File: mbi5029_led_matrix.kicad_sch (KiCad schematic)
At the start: 19 parts, among them Q1 pCh SO23, Q10 pCh SO23, Q11 pCh SO23, Q12 pCh SO23, Q13 pCh SO23, Q14 pCh SO23, Q15 pCh SO23, Q16 pCh SO23, Q2 pCh SO23, Q3 pCh SO23, Q4 pCh SO23, Q5 pCh SO23, Q6 pCh SO23, Q7 pCh SO23, Q8 pCh SO23, Q9 pCh SO23, U1 MBI5029, U2 74HC237, U3 74HC237

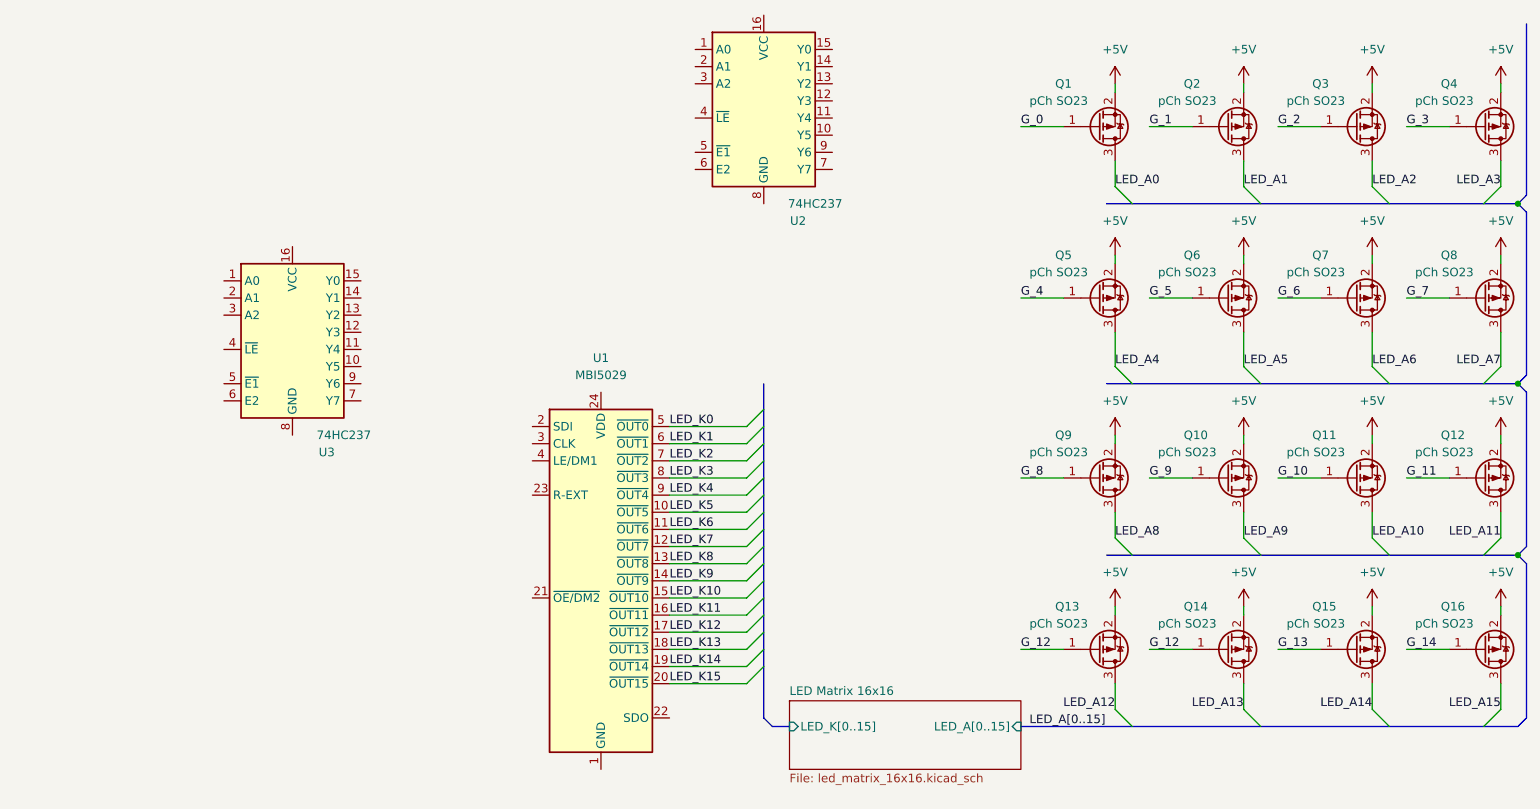
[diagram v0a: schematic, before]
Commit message: work
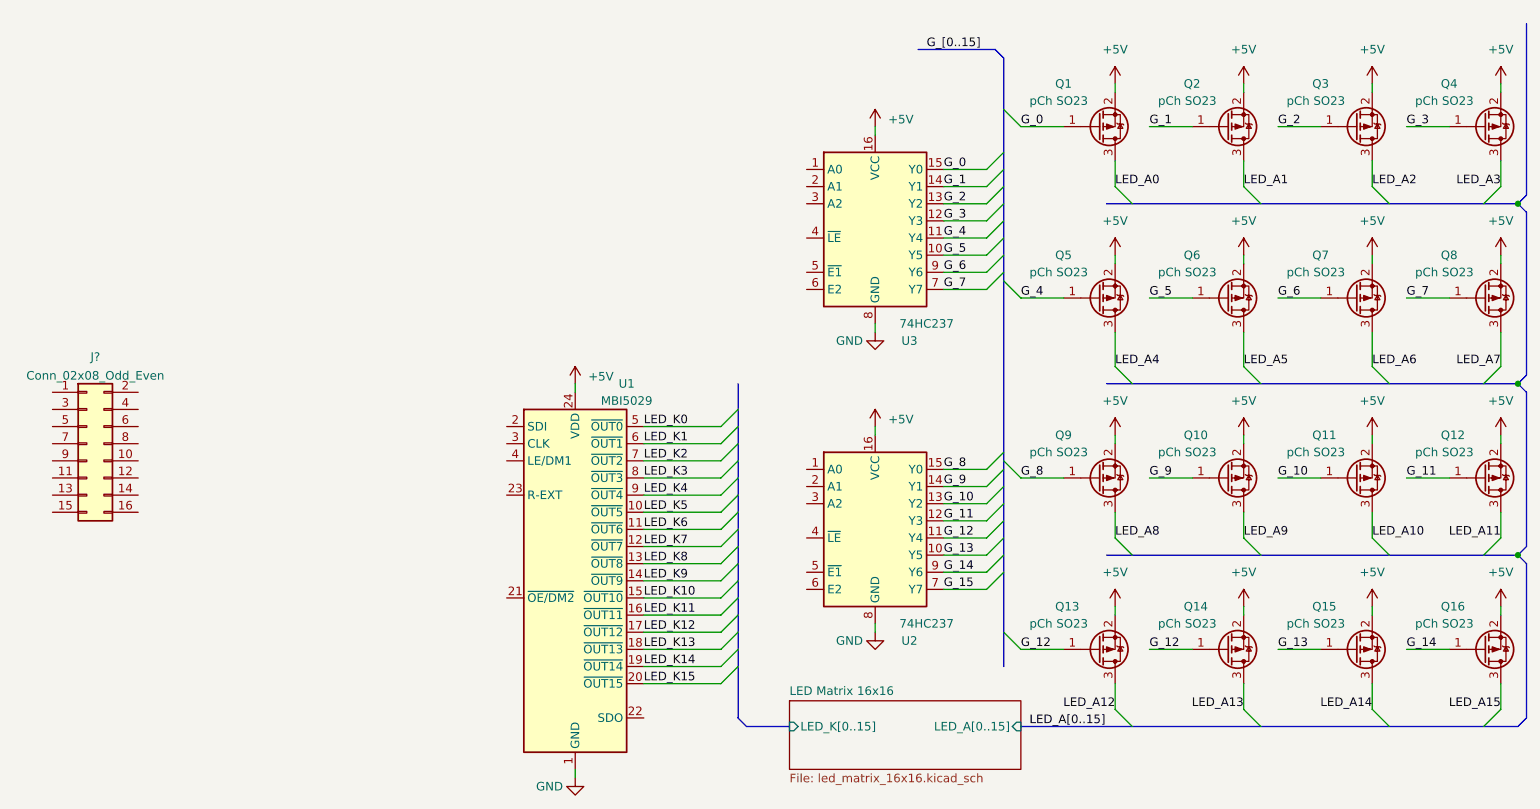
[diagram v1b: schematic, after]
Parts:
- added J?: Conn_02x08_Odd_Even, symbol Connector_Generic:Conn_02x08_Odd_Even
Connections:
- net +5V: now also U1.24 (VDD), U2.16 (VCC), U3.16 (VCC)
- net G_0: now also U3.15 (Y0)
- net G_1: now also U3.14 (Y1)
- net G_10: now also U2.13 (Y2)
- net G_11: now also U2.12 (Y3)
- net G_12: now also U2.11 (Y4)
- net G_13: now also U2.10 (Y5)
- net G_14: now also U2.9 (Y6)
- net G_2: now also U3.13 (Y2)
- net G_3: now also U3.12 (Y3)
- net G_4: now also U3.11 (Y4)
- net G_5: now also U3.10 (Y5)
- net G_6: now also U3.9 (Y6)
- net G_7: now also U3.7 (Y7)
- net G_8: now also U2.15 (Y0)
- net G_9: now also U2.14 (Y1)
- net GND: now reaches U3.8 (GND)
- net GND: now also U1.1 (GND), U2.8 (GND)
- net G_15: now reaches U2.7 (Y7)
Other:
- moved on the sheet: U1, U2, U3
